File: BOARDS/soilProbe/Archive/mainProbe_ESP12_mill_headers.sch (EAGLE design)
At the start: 18 parts

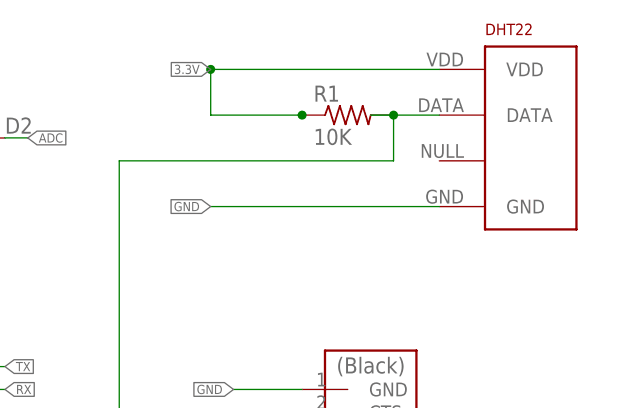
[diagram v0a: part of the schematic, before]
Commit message: new data
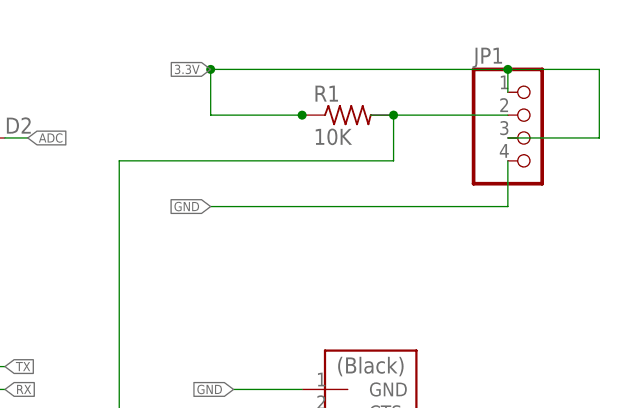
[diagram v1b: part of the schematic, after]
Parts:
- removed DHT22: (no value), RHT03_DHT-22_AM2302:RHT03_DHT-22_AM2302
- added JP1: (no value), pinhead:PINHD-1X4
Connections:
- net 3.3V: now also JP1.1, JP1.3; no longer DHT22.VDD
- net GND: now also JP1.4; no longer DHT22.GND
- net N$8: now also JP1.2; no longer DHT22.DATA
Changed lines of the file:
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@@
 <part name="D1" library="fab" deviceset="DIODE" device="SOD123"/>
 <part name="D2" library="fab" deviceset="DIODE" device="SOD123"/>
-<part name="DHT22" library="RHT03_DHT-22_AM2302" deviceset="RHT03_DHT-22_AM2302" device=""/>
 <part name="R2" library="fab" deviceset="RES-US" device="1206" value="4.7K"/>
 <part name="R3" library="fab" deviceset="RES-US" device="1206" value="10k"/>
@@
 <part name="TEMPSENSOR" library="pinhead" library_urn="urn:adsk.eagle:library:325" deviceset="PINHD-1X3" device="" package3d_urn="urn:adsk.eagle:package:22458/2"/>
 <part name="SOLARIN" library="pinhead" library_urn="urn:adsk.eagle:library:325" deviceset="PINHD-1X2" device="/90" package3d_urn="urn:adsk.eagle:package:22437/2"/>
+<part name="JP1" library="pinhead" library_urn="urn:adsk.eagle:library:325" deviceset="PINHD-1X4" device="" package3d_urn="urn:adsk.eagle:package:22407/2"/>
 </parts>
 <sheets>
@@
 <instance part="D1" gate="G$1" x="68.58" y="83.82"/>
 <instance part="D2" gate="G$1" x="96.52" y="83.82"/>
-<instance part="DHT22" gate="G$1" x="157.48" y="83.82"/>
 <instance part="R2" gate="G$1" x="30.48" y="48.26" rot="R90"/>
 <instance part="R3" gate="G$1" x="63.5" y="81.28" rot="R90"/>
@@
 <instance part="TEMPSENSOR" gate="A" x="20.32" y="58.42" rot="R180"/>
 <instance part="SOLARIN" gate="G$1" x="91.44" y="25.4" rot="R180"/>
+<instance part="JP1" gate="A" x="157.48" y="83.82"/>
 </instances>
 <busses>
@@
 <net name="N$8" class="0">
 <segment>
-<pinref part="DHT22" gate="G$1" pin="DATA"/>
-<wire x1="147.32" y1="86.36" x2="142.24" y2="86.36" width="0.1524" layer="91"/>
 <pinref part="R1" gate="G$1" pin="2"/>
 <wire x1="142.24" y1="86.36" x2="139.7" y2="86.36" width="0.1524" layer="91"/>
@@
 <wire x1="111.76" y1="45.72" x2="93.98" y2="45.72" width="0.1524" layer="91"/>
 <junction x="93.98" y="45.72"/>
+<pinref part="JP1" gate="A" pin="2"/>
+<wire x1="142.24" y1="86.36" x2="154.94" y2="86.36" width="0.1524" layer="91"/>
 </segment>
 </net>
@@
 </segment>
 <segment>
-<pinref part="DHT22" gate="G$1" pin="GND"/>
-<wire x1="147.32" y1="76.2" x2="121.92" y2="76.2" width="0.1524" layer="91"/>
+<wire x1="154.94" y1="76.2" x2="121.92" y2="76.2" width="0.1524" layer="91"/>
 <label x="121.92" y="76.2" size="1.016" layer="95" rot="R180" xref="yes"/>
+<pinref part="JP1" gate="A" pin="4"/>
+<wire x1="154.94" y1="76.2" x2="154.94" y2="81.28" width="0.1524" layer="91"/>
 </segment>
 <segment>
@@
 </segment>
 <segment>
-<pinref part="DHT22" gate="G$1" pin="VDD"/>
-<wire x1="147.32" y1="91.44" x2="121.92" y2="91.44" width="0.1524" layer="91"/>
+<wire x1="154.94" y1="91.44" x2="121.92" y2="91.44" width="0.1524" layer="91"/>
 <label x="121.92" y="91.44" size="1.016" layer="95" rot="R180" xref="yes"/>
 <pinref part="R1" gate="G$1" pin="1"/>
@@
 <junction x="121.92" y="91.44"/>
 <junction x="132.08" y="86.36"/>
-</segment>
-<segment>
+<pinref part="JP1" gate="A" pin="1"/>
+<wire x1="154.94" y1="91.44" x2="154.94" y2="88.9" width="0.1524" layer="91"/>
+<wire x1="154.94" y1="91.44" x2="165.1" y2="91.44" width="0.1524" layer="91"/>
+<wire x1="165.1" y1="91.44" x2="165.1" y2="83.82" width="0.1524" layer="91"/>
+<junction x="154.94" y="91.44"/>
+<pinref part="JP1" gate="A" pin="3"/>
+<wire x1="165.1" y1="83.82" x2="154.94" y2="83.82" width="0.1524" layer="91"/>
+</segment>
+<segment>
